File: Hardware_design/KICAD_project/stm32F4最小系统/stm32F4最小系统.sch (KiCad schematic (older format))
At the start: 2 parts

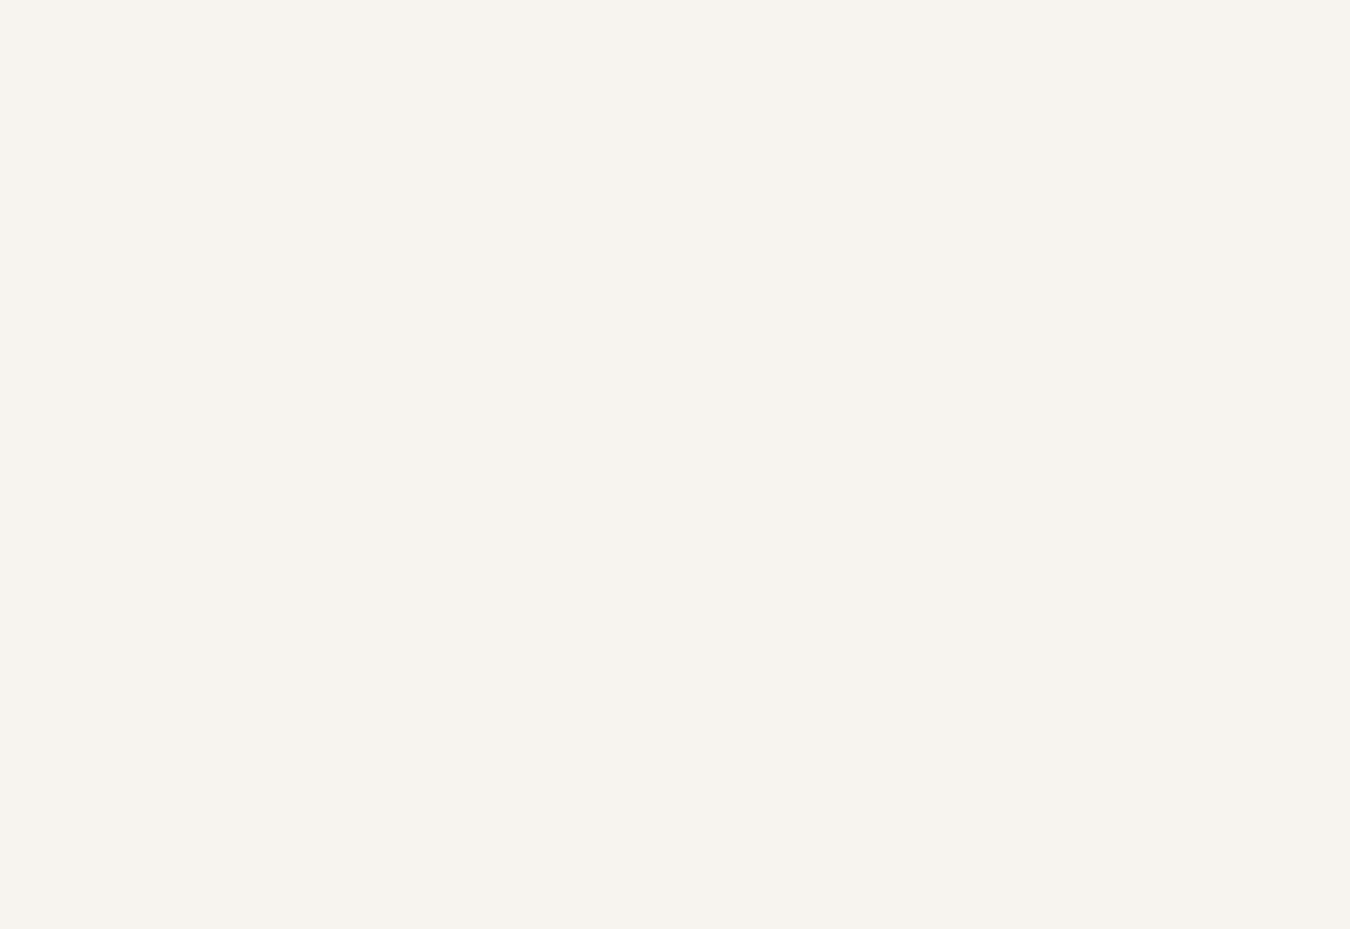
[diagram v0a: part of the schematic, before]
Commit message: BMI088
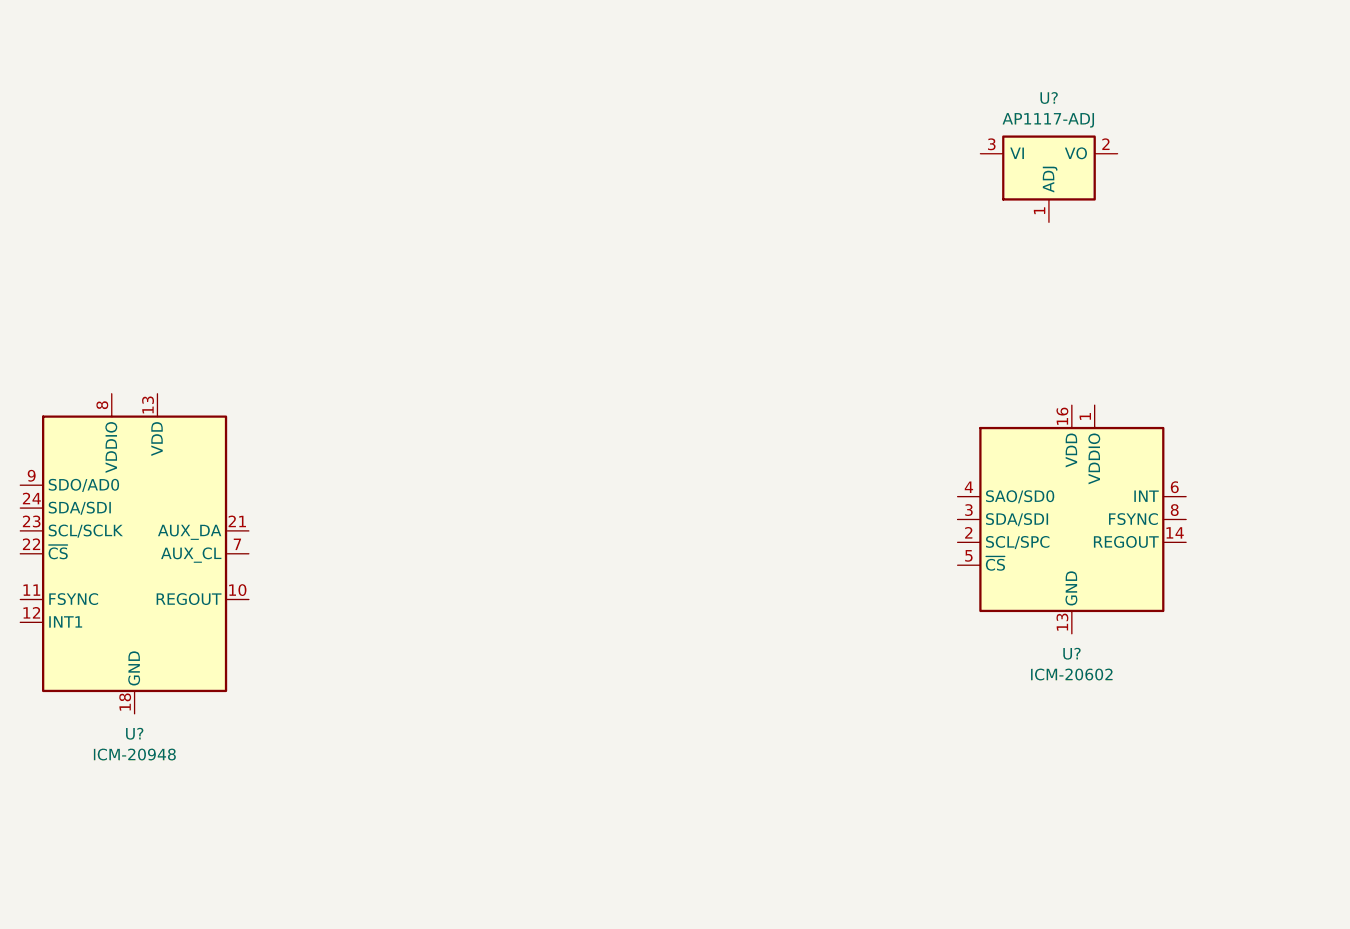
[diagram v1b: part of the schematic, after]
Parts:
- added U?: AP1117-ADJ, Package_TO_SOT_SMD:SOT-223-3_TabPin2, symbol Regulator_Linear:AP1117-ADJ
- added U?: ICM-20602, Package_LGA:LGA-16_3x3mm_P0.5mm_LayoutBorder3x5y, symbol Sensor_Motion:ICM-20602
- added U?: ICM-20948, Sensor_Motion:InvenSense_QFN-24_3x3mm_P0.4mm, symbol Sensor_Motion:ICM-20948
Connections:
- new net: U?.10 (GND), U?.11 (GND), U?.12 (GND), U?.13 (GND), U?.15 (GND), U?.9 (GND)
- new net: U?.18 (GND), U?.20 (GND)
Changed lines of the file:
@@
+	1    0    0    -1
+$EndComp
+$Comp
+L Regulator_Linear:AP1117-ADJ U?
+U 1 1 6021629F
+P 9550 5150
+F 0 "U?" H 9550 5392 50  0000 C CNN
+F 1 "AP1117-ADJ" H 9550 5301 50  0000 C CNN
+F 2 "Package_TO_SOT_SMD:SOT-223-3_TabPin2" H 9550 5350 50  0001 C CNN
+F 3 "http://www.diodes.com/datasheets/AP1117.pdf" H 9650 4900 50  0001 C CNN
+	1    9550 5150
+	1    0    0    -1
+$EndComp
+$Comp
+L Sensor_Motion:ICM-20602 U?
+U 1 1 60216D37
+P 9650 6750
+F 0 "U?" H 9650 6161 50  0000 C CNN
+F 1 "ICM-20602" H 9650 6070 50  0000 C CNN
+F 2 "Package_LGA:LGA-16_3x3mm_P0.5mm_LayoutBorder3x5y" H 9650 7000 50  0001 C CNN
+F 3 "http://www.invensense.com/wp-content/uploads/2016/10/DS-000176-ICM-20602-v1.0.pdf" H 9700 7700 50  0001 C CNN
+	1    9650 6750
+	1    0    0    -1
+$EndComp
+$Comp
+L Sensor_Motion:ICM-20948 U?
+U 1 1 60218B58
+P 5550 6900
+F 0 "U?" H 5550 6111 50  0000 C CNN
+F 1 "ICM-20948" H 5550 6020 50  0000 C CNN
+F 2 "Sensor_Motion:InvenSense_QFN-24_3x3mm_P0.4mm" H 5550 5900 50  0001 C CNN
+F 3 "http://www.invensense.com/wp-content/uploads/2016/06/DS-000189-ICM-20948-v1.3.pdf" H 5550 6750 50  0001 C CNN
+	1    5550 6900
 	1    0    0    -1
 $EndComp
